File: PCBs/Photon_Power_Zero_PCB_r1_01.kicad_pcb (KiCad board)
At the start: 2 copper layers, 65.1 x 30.1 mm, 56 parts, among them J1 JST_S2B-PH-SM4-TB_LF__SN_, J2 JST_GH_SM02B-GHS-TB_1x02-1MP_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, J3 SMT_Solar_barrel, U1 ATtiny84-SSFR, U2 REG_MCP1700T-3602E/MB, U3 bq2407, U4 AP2161-WG, U5 TPS613222A

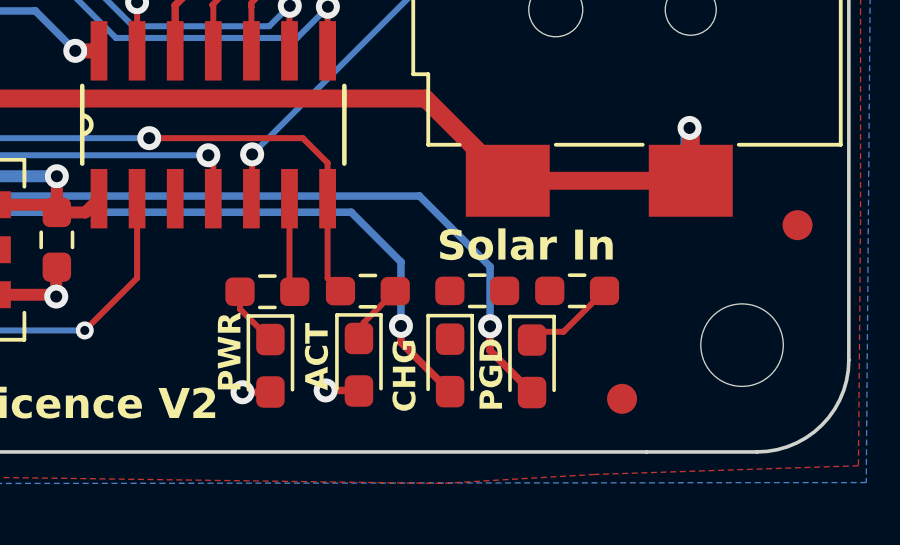
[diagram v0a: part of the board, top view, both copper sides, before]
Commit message: changes for rev2 and cleanup
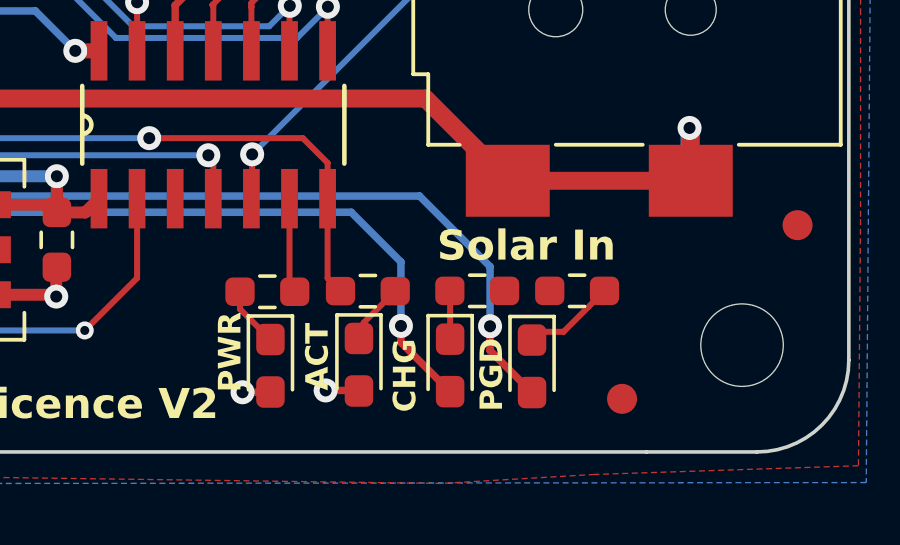
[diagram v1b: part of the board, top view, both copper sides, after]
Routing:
- net (no net): track 391.5 -> 393.1 mm
